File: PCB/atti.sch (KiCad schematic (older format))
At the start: 4 parts

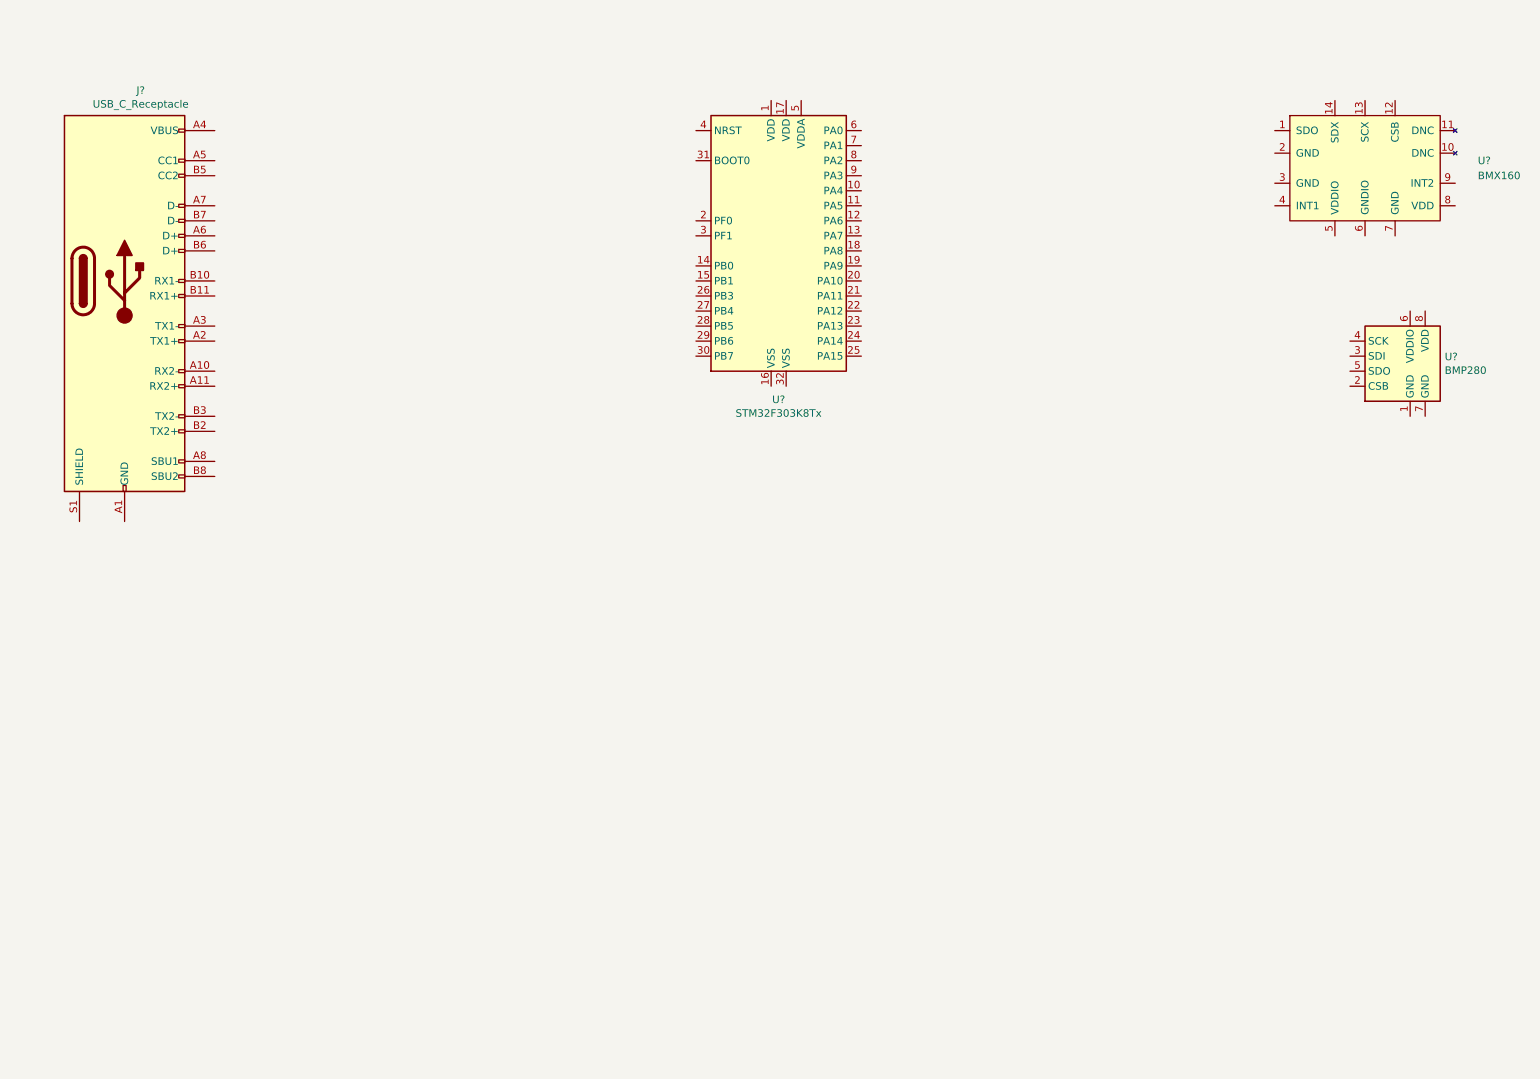
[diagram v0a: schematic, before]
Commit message: Preliminary subdesign
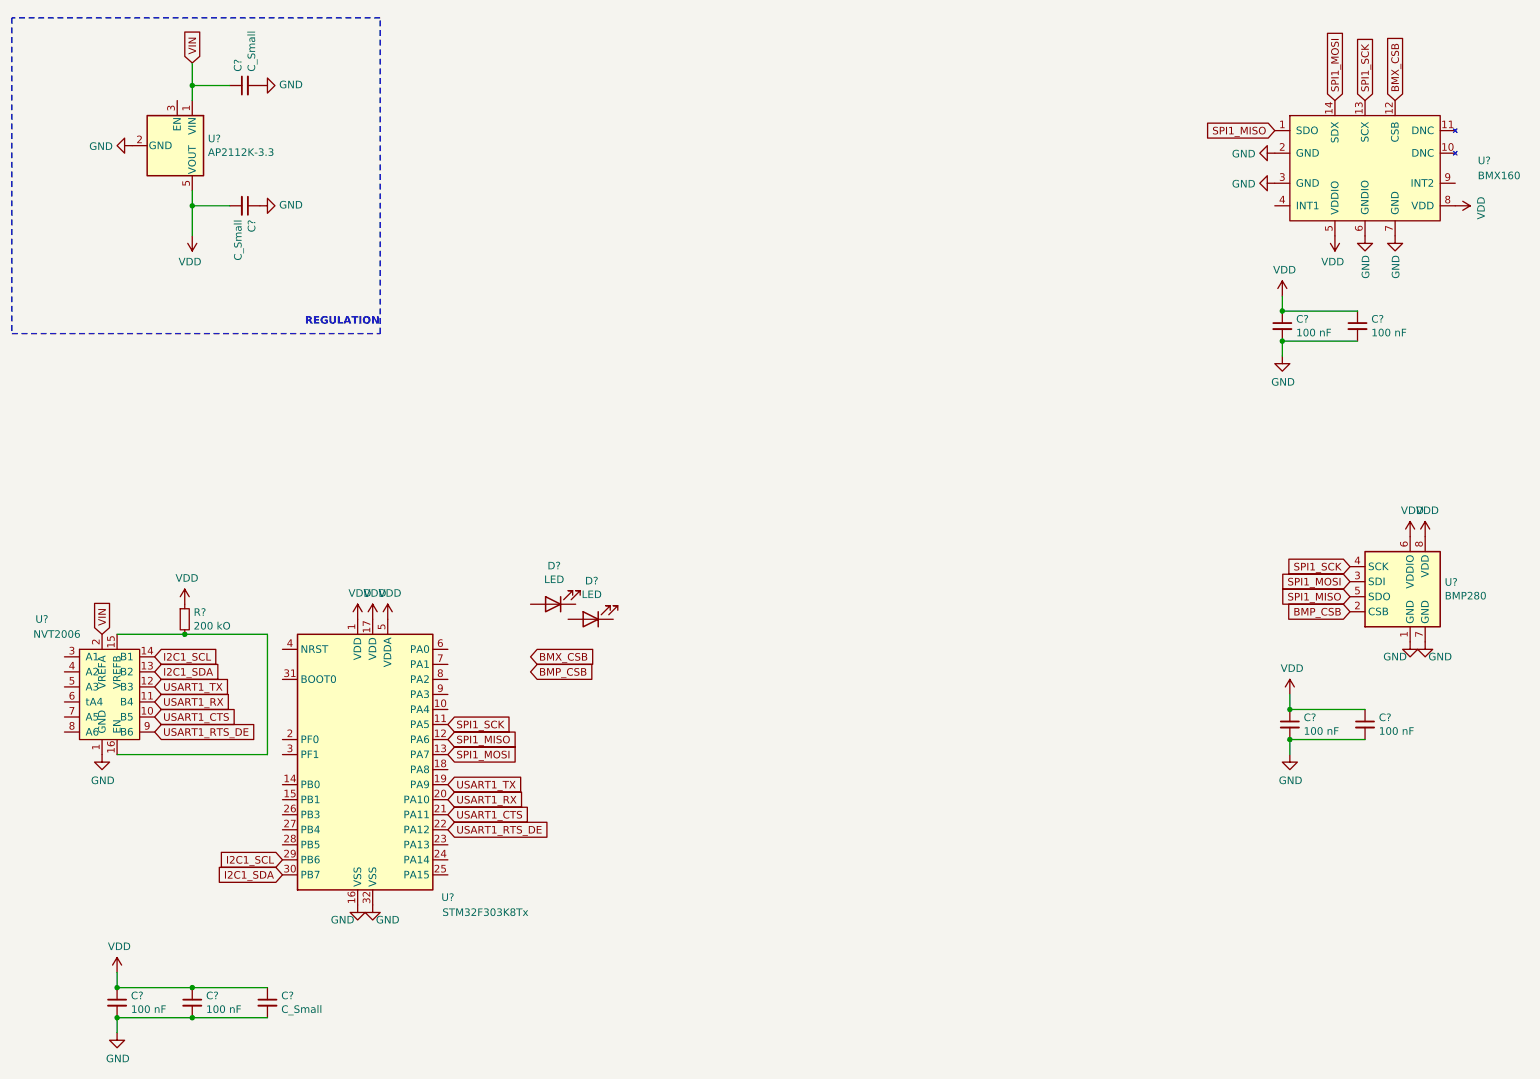
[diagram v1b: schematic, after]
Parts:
- removed J?: USB_C_Receptacle, symbol Connector:USB_C_Receptacle
- added C? (x3): C_Small, symbol Device:C_Small
- added C? (x6): 100 nF, symbol Device:C_Small
- added D? (x2): LED, symbol Device:LED
- added R?: 200 kO, symbol Device:R_Small
- added U?: AP2112K-3.3, Package_TO_SOT_SMD:SOT-23-5, symbol Regulator_Linear:AP2112K-3.3
- added U?: NVT2006, symbol AsymLevelShifters:NVT2006
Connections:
- net SPI1_MISO: now reaches U?.1 (SDO)
- net SPI1_MISO: now also U?.12 (PA6), U?.5 (SDO)
- net BMX_CSB: now reaches U?.12 (CSB)
- net SPI1_SCK: now reaches U?.13 (SCX)
- net SPI1_SCK: now also U?.11 (PA5), U?.4 (SCK)
- net SPI1_MOSI: now reaches U?.14 (SDX)
- net SPI1_MOSI: now also U?.13 (PA7), U?.3 (SDI)
- net GND: now reaches U?.2 (GND)
- net GND: now also U?.1 (GND), U?.16 (VSS), U?.3 (GND), U?.32 (VSS), U?.6 (GNDIO), U?.7 (GND), U?.7 (GND), C?.1, C?.2, C?.2, C?.2, C?.2, C?.2, C?.2, C?.2, C?.2, U?.1 (GND), U?.2 (GND)
- net VDD: now reaches U?.5 (VDDIO)
- net VDD: now also U?.1 (VDD), U?.17 (VDD), U?.5 (VDDA), U?.6 (VDDIO), U?.8 (VDD), U?.8 (VDD), C?.1, C?.1, C?.1, C?.1, C?.1, C?.1, C?.1, C?.2, R?.1, U?.5 (VOUT)
- net BMP_CSB: now reaches U?.2 (CSB)
- net USART1_TX: now reaches U?.19 (PA9)
- net USART1_TX: now also U?.12 (B3)
- net USART1_RX: now reaches U?.20 (PA10)
- net USART1_RX: now also U?.11 (B4)
- net USART1_CTS: now reaches U?.21 (PA11)
- net USART1_CTS: now also U?.10 (B5)
- net USART1_RTS_DE: now reaches U?.22 (PA12)
- net USART1_RTS_DE: now also U?.9 (B6)
- net I2C1_SCL: now reaches U?.29 (PB6)
- net I2C1_SCL: now also U?.14 (B1)
- net I2C1_SDA: now reaches U?.30 (PB7)
- net I2C1_SDA: now also U?.13 (B2)
- new net: R?.2, U?.15 (VREFB), U?.16 (EN)
- new net VIN: C?.1, U?.1 (VIN), U?.2 (VREFA)
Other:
- note added: "REGULATION"
- moved on the sheet: U?
